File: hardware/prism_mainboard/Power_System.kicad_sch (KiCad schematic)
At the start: 72 parts, among them U4 AMS1117-1.8, U5 AMS1117-1.8, U6 AMS1117-1.8, U7 AMS1117-1.8

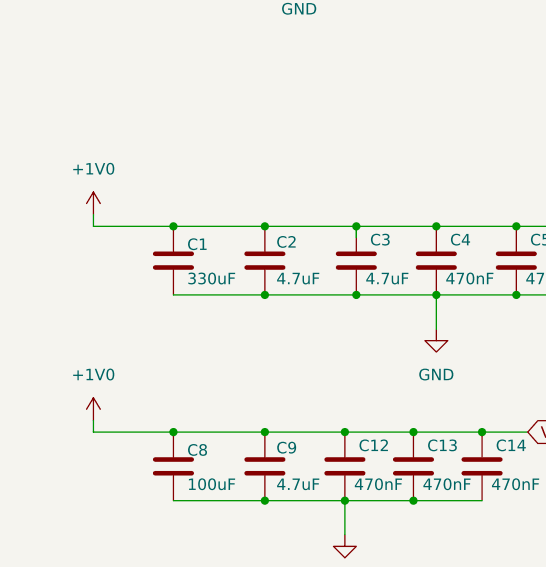
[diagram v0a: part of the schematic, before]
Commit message: Updates
Mostly Schematic updates, nothing too big. Added a few datasheets
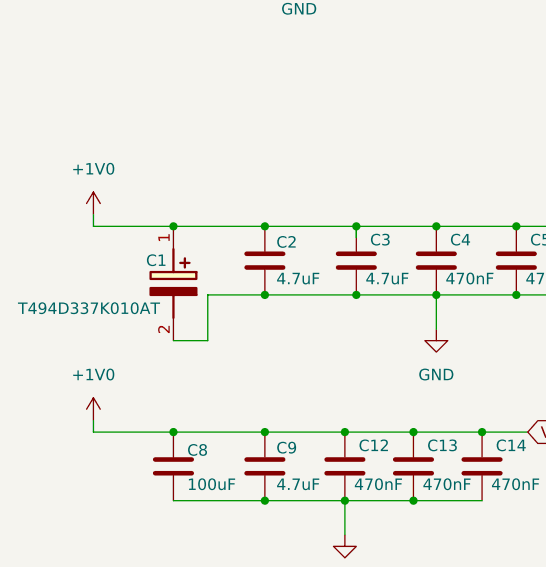
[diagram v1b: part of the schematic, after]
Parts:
- removed C1: 330uF, symbol Device:C
- added C1: T494D337K010AT, T494D, symbol SamacSys:T494D337K010AT
- R1, R2, R3, R4: footprint (none) -> Resistor_SMD:R_0805_2012Metric_Pad1.20x1.40mm_HandSolder
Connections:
- net +1V0: now also C1.1 (+)
- net GND: now also C1.2 (-)
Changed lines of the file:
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@@
 	(wire
 		(pts
-			(xy 171.45 48.26) (xy 171.45 50.8)
+			(xy 38.1 96.52) (xy 38.1 91.44)
 		)
 		(stroke
@@
 	(wire
 		(pts
-			(xy 48.26 39.37) (xy 53.34 39.37)
+			(xy 171.45 48.26) (xy 171.45 50.8)
 		)
 		(stroke
@@
 	(wire
 		(pts
-			(xy 30.48 163.83) (xy 35.56 163.83)
+			(xy 48.26 39.37) (xy 53.34 39.37)
 		)
 		(stroke
@@
 	(wire
 		(pts
-			(xy 229.87 69.85) (xy 237.49 69.85)
+			(xy 30.48 163.83) (xy 35.56 163.83)
 		)
 		(stroke
@@
 	(wire
 		(pts
-			(xy 58.42 39.37) (xy 67.31 39.37)
+			(xy 229.87 69.85) (xy 237.49 69.85)
 		)
 		(stroke
@@
 	(wire
 		(pts
-			(xy 251.46 115.57) (xy 259.08 115.57)
+			(xy 58.42 39.37) (xy 67.31 39.37)
 		)
 		(stroke
@@
 	(wire
 		(pts
-			(xy 34.29 91.44) (xy 44.45 91.44)
+			(xy 251.46 115.57) (xy 259.08 115.57)
 		)
 		(stroke
@@
 	(wire
 		(pts
+			(xy 38.1 91.44) (xy 44.45 91.44)
+		)
+		(stroke
+			(width 0)
+			(type default)
+		)
+	)
+	(wire
+		(pts
 			(xy 195.58 40.64) (xy 204.47 40.64)
 		)
@@
 	(wire
 		(pts
+			(xy 34.29 96.52) (xy 38.1 96.52)
+		)
+		(stroke
+			(width 0)
+			(type default)
+		)
+	)
+	(wire
+		(pts
 			(xy 116.84 140.97) (xy 125.73 140.97)
 		)
@@
 			)
 		)
-		(property "Footprint" ""
+		(property "Footprint" "Resistor_SMD:R_0805_2012Metric_Pad1.20x1.40mm_HandSolder"
 			(at 193.802 44.45 90)
 			(hide yes)
@@
 			)
 		)
-		(property "Footprint" ""
+		(property "Footprint" "Resistor_SMD:R_0805_2012Metric_Pad1.20x1.40mm_HandSolder"
 			(at 193.802 31.75 90)
 			(hide yes)
@@
 			)
 		)
-		(property "Footprint" ""
+		(property "Footprint" "Resistor_SMD:R_0805_2012Metric_Pad1.20x1.40mm_HandSolder"
 			(at 169.672 44.45 90)
 			(hide yes)
@@
 			)
 		)
-		(property "Footprint" ""
+		(property "Footprint" "Resistor_SMD:R_0805_2012Metric_Pad1.20x1.40mm_HandSolder"
 			(at 169.672 31.75 90)
 			(hide yes)
@@
 	)
 	(symbol
+		(lib_id "SamacSys:T494D337K010AT")
+		(at 34.29 83.82 270)
+		(unit 1)
+		(body_style 1)
+		(exclude_from_sim no)
+		(in_bom yes)
+		(on_board yes)
+		(in_pos_files yes)
+		(dnp no)
+		(property "Reference" "C1"
+			(at 31.242 87.63 90)
+			(show_name no)
+			(do_not_autoplace no)
+			(effects
+				(font
+					(size 1.27 1.27)
+				)
+				(justify left)
+			)
+		)
+		(property "Value" "T494D337K010AT"
+			(at 17.018 92.964 90)
+			(show_name no)
+			(do_not_autoplace no)
+			(effects
+				(font
+					(size 1.27 1.27)
+				)
+				(justify left)
+			)
+		)
+		(property "Footprint" "T494D"
+			(at -61.9 92.71 0)
+			(hide yes)
+			(show_name no)
+			(do_not_autoplace no)
+			(effects
+				(font
+					(size 1.27 1.27)
+				)
+				(justify left top)
+			)
+		)
+		(property "Datasheet" "https://www.yageogroup.com/content/datasheet/asset/file/KEM_T2008_T494"
+			(at -161.9 92.71 0)
+			(hide yes)
+			(show_name no)
+			(do_not_autoplace no)
+			(effects
+				(font
+					(size 1.27 1.27)
+				)
+				(justify left top)
+			)
+		)
+		(property "Description" "SMD, MnO2, Molded, Low ESR"
+			(at 34.29 83.82 0)
+			(hide yes)
+			(show_name no)
+			(do_not_autoplace no)
+			(effects
+				(font
+					(size 1.27 1.27)
+				)
+			)
+		)
+		(property "Height" "3.1"
+			(at -361.9 92.71 0)
+			(hide yes)
+			(show_name no)
+			(do_not_autoplace no)
+			(effects
+				(font
+					(size 1.27 1.27)
+				)
+				(justify left top)
+			)
+		)
+		(property "Manufacturer_Name" "Yageo Group"
+			(at -461.9 92.71 0)
+			(hide yes)
+			(show_name no)
+			(do_not_autoplace no)
+			(effects
+				(font
+					(size 1.27 1.27)
+				)
+				(justify left top)
+			)
+		)
+		(property "Manufacturer_Part_Number" "T494D337K010AT"
+			(at -561.9 92.71 0)
+			(hide yes)
+			(show_name no)
+			(do_not_autoplace no)
+			(effects
+				(font
+					(size 1.27 1.27)
+				)
+				(justify left top)
+			)
+		)
+		(property "Mouser Part Number" "80-T494D337K010AT"
+			(at -661.9 92.71 0)
+			(hide yes)
+			(show_name no)
+			(do_not_autoplace no)
+			(effects
+				(font
+					(size 1.27 1.27)
+				)
+				(justify left top)
+			)
+		)
+		(property "Mouser Price/Stock" "https://www.mouser.co.uk/ProductDetail/KEMET/T494D337K010AT?qs=AaRlLUpeMszja%252B890bVUVg%3D%3D"
+			(at -761.9 92.71 0)
+			(hide yes)
+			(show_name no)
+			(do_not_autoplace no)
+			(effects
+				(font
+					(size 1.27 1.27)
+				)
+				(justify left top)
+			)
+		)
+		(property "Arrow Part Number" "T494D337K010AT"
+			(at -861.9 92.71 0)
+			(hide yes)
+			(show_name no)
+			(do_not_autoplace no)
+			(effects
+				(font
+					(size 1.27 1.27)
+				)
+				(justify left top)
+			)
+		)
+		(property "Arrow Price/Stock" "https://www.arrow.com/en/products/t494d337k010at/kemet-corporation"
+			(at -961.9 92.71 0)
+			(hide yes)
+			(show_name no)
+			(do_not_autoplace no)
+			(effects
+				(font
+					(size 1.27 1.27)
+				)
+				(justify left top)
+			)
+		)
+		(pin "1"
+		)
+		(pin "2"
+		)
+		(instances
+			(project "prism_mainboard"
+				(path "/1d5f25f9-3e6f-41df-a8ec-41fc885bea9a/2fdb70e6-73b6-44a0-9464-64831d844f2c"
+					(reference "C1")
+					(unit 1)
+				)
+			)
+		)
+	)
+	(symbol
 		(lib_id "power:GND")
 		(at 53.34 118.11 0)
@@
 					(unit 1)
 				)
-			)
-		)
-	)
-	(symbol
-		(lib_id "Device:C")
-		(at 34.29 87.63 0)
-		(unit 1)
-		(body_style 1)
-		(exclude_from_sim no)
-		(in_bom yes)
-		(on_board yes)
-		(in_pos_files yes)
-		(dnp no)
-		(property "Reference" "C1"
-			(at 35.814 85.852 0)
-			(show_name no)
-			(do_not_autoplace no)
-			(effects
-				(font
-					(size 1.27 1.27)
-				)
-				(justify left)
-			)
-		)
-		(property "Value" "330uF"
-			(at 35.814 89.662 0)
-			(show_name no)
-			(do_not_autoplace no)
-			(effects
-				(font
-					(size 1.27 1.27)
-				)
-				(justify left)
-			)
-		)
-		(property "Footprint" ""
-			(at 35.2552 91.44 0)
-			(hide yes)
-			(show_name no)
-			(do_not_autoplace no)
-			(effects
-				(font
-					(size 1.27 1.27)
-				)
-			)
-		)
-		(property "Datasheet" ""
-			(at 34.29 87.63 0)
-			(hide yes)
-			(show_name no)
-			(do_not_autoplace no)
-			(effects
-				(font
-					(size 1.27 1.27)
-				)
-			)
-		)
-		(property "Description" "Unpolarized capacitor"
-			(at 34.29 87.63 0)
-			(hide yes)
-			(show_name no)
-			(do_not_autoplace no)
-			(effects
-				(font
-					(size 1.27 1.27)
-				)
-			)
-		)
-		(pin "1"
-		)
-		(pin "2"
-		)
-		(instances
-			(project "prism_mainboard"
-				(path "/1d5f25f9-3e6f-41df-a8ec-41fc885bea9a/2fdb70e6-73b6-44a0-9464-64831d844f2c"
-					(reference "C1")
-					(unit 1)
-				)
